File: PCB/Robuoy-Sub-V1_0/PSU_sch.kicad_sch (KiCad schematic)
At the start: 27 parts, among them U1 TPS5430DDAR, U7 TLV61046ADB, U8 TLV61046ADB

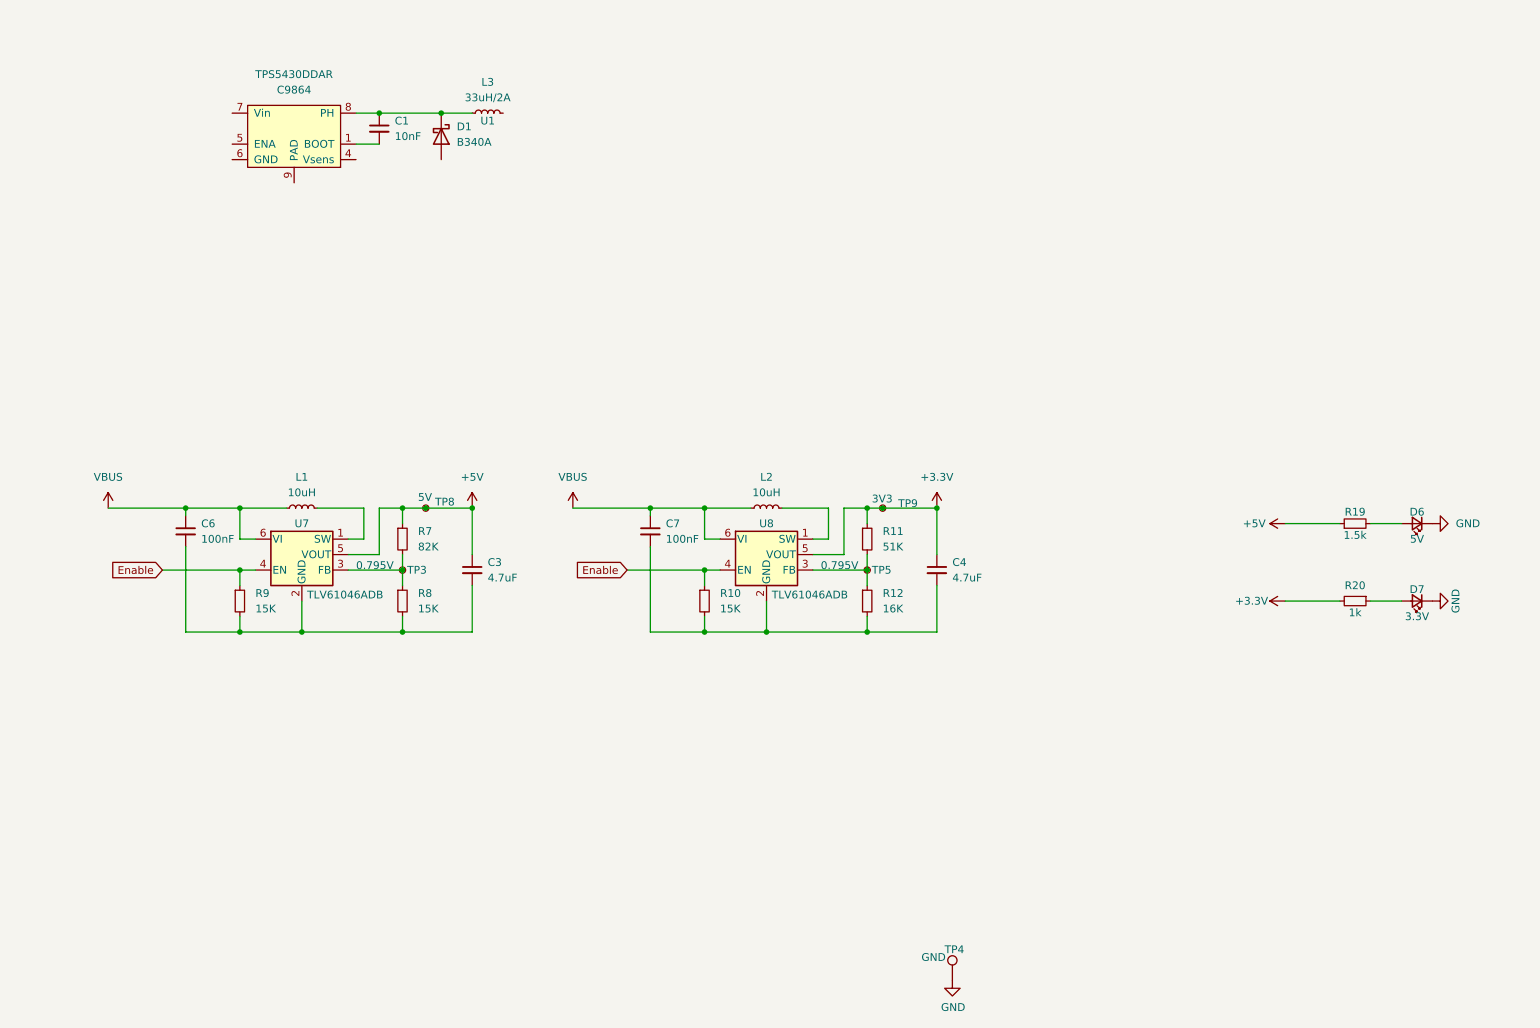
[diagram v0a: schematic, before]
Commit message: Schematic changes not yet finished!
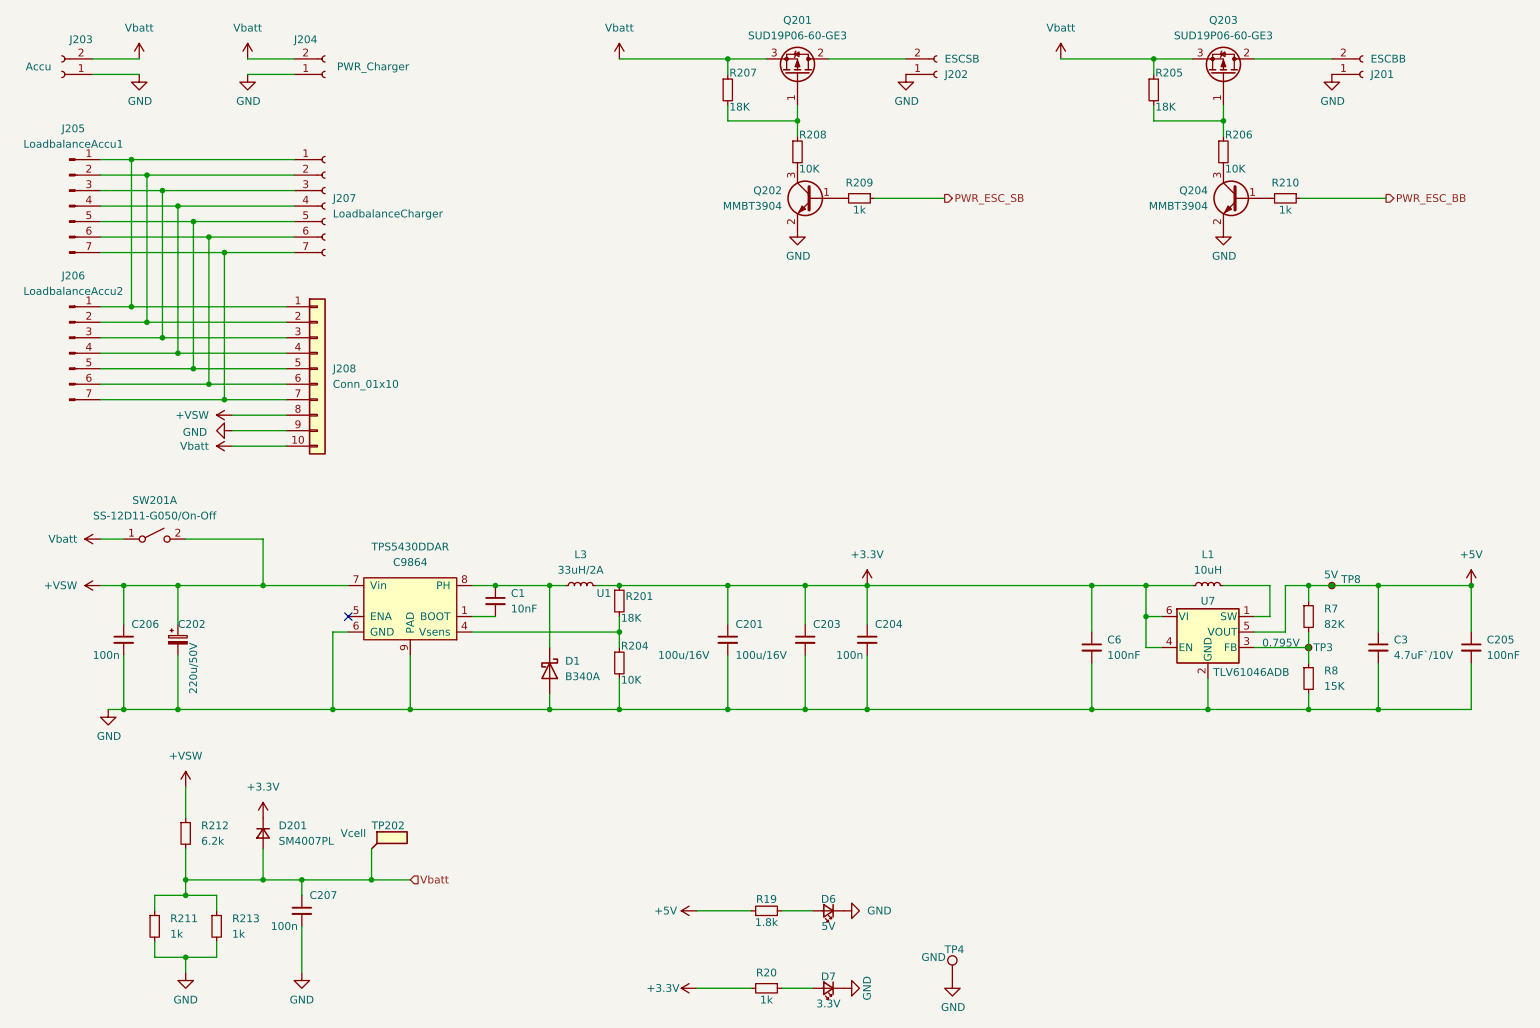
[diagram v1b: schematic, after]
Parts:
- removed C4: 4.7uF, symbol Device:C_Small
- removed C7: 100nF, symbol Device:C_Small
- removed L2: 10uH, symbol Device:L_Small
- removed R10, R9: 15K, symbol Device:R_Small
- removed R11: 51K, symbol Device:R_Small
- removed R12: 16K, symbol Device:R_Small
- removed TP5: 0.795V, symbol Connector:TestPoint_Small
- removed TP9: 3V3, symbol Connector:TestPoint_Small
- removed U8: TLV61046ADB, Package_TO_SOT_SMD:SOT-23-6, symbol Regulator_Switching:TLV61046ADB
- added C201, C203: 100u/16V, Capacitor_SMD:C_1210_3225Metric, symbol Device:C_Small
- added C202: 220u/50V, A_Device:CP_ALU_D10x10.5, symbol Device:C_Polarized_Small
- added C204, C206, C207: 100n, A_Device:C_0603, symbol Device:C_Small
- added C205: 100nF, symbol Device:C_Small
- added D201: SM4007PL, A_Device:D_SOD-123_2.85x1.8x1.3, symbol Device:D_Small
- added J201: ESCBB, symbol Connector:Conn_01x02_Socket
- added J202: ESCSB, symbol Connector:Conn_01x02_Socket
- added J203: Accu, A_Connector:AMASS_XT60-M_1x02_P7.20mm_Vertical, symbol Connector:Conn_01x02_Socket
- added J204: PWR_Charger, A_Connector:AMASS_XT60-M_1x02_P7.20mm_Vertical, symbol Connector:Conn_01x02_Socket
- added J205: LoadbalanceAccu1, symbol Connector:Conn_01x07_Pin
- added J206: LoadbalanceAccu2, symbol Connector:Conn_01x07_Pin
- added J207: LoadbalanceCharger, symbol Connector:Conn_01x07_Socket
- added J208: Conn_01x10, symbol Connector_Generic:Conn_01x10
- added Q201, Q203: SUD19P06-60-GE3, Package_TO_SOT_SMD:TO-252-2, symbol Transistor_FET:SUD19P06-60
- added Q202, Q204: MMBT3904, Package_TO_SOT_SMD:SOT-23, symbol Transistor_BJT:MMBT3904
- added R201, R205, R207: 18K, symbol Device:R_Small
- added R204, R206, R208: 10K, symbol Device:R_Small
- added R209, R210, R211, R213: 1k, A_Device:R_0603, symbol Device:R_Small
- added R212: 6.2k, A_Device:R_0603, symbol Device:R_Small
- added SW201: SS-12D11-G050/On-Off, symbol Switch:SW_DPST_x2
- added TP202: Vcell, A_Pads_Pins:Testpoint_0.6x1.0, symbol Connector:TestPoint_Flag
- C3: value 4.7uF -> 4.7uF`/10V
- R19: value 1.5k -> 1.8k; LCSC C22843 -> (none)
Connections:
- net Enable is gone; now on net +3.3V: U7.4 (EN)
- net VBUS is gone; now on net +3.3V: C6.1, L1.1, U7.6 (VI)
- net +3.3V: now also L3.2, C201.1, C203.1, C204.1, D201.1 (K), R201.1
- net +5V: now also C205.1
- net GND: now also C3.2, C6.2, D1.2 (A), R8.2, U1.6 (GND), U1.9 (PAD), U7.2 (GND), C201.2, C202.2, C203.2, C204.2, C205.2, C206.2, C207.2, J201.1 (Pin_1), J202.1 (Pin_1), J203.1 (Pin_1), J204.1 (Pin_1), J208.9 (Pin_9), Q202.2 (E), Q204.2 (E), R204.2, R211.2, R213.2
- net at U1.4 (Vsens): now also R201.2, R204.1
- net +VSW: now reaches U1.7 (Vin)
- net +VSW: now also C202.1, C206.1, J208.8 (Pin_8), R212.1, SW201.2 (B)
- new net: J201.2 (Pin_2), Q203.2 (D)
- new net: Q204.1 (B), R210.2
- new net: J205.1 (Pin_1), J206.1 (Pin_1), J207.1 (Pin_1), J208.1 (Pin_1)
- new net: J205.2 (Pin_2), J206.2 (Pin_2), J207.2 (Pin_2), J208.2 (Pin_2)
- new net: J205.3 (Pin_3), J206.3 (Pin_3), J207.3 (Pin_3), J208.3 (Pin_3)
- new net: J205.4 (Pin_4), J206.4 (Pin_4), J207.4 (Pin_4), J208.4 (Pin_4)
- new net: J205.5 (Pin_5), J206.5 (Pin_5), J207.5 (Pin_5), J208.5 (Pin_5)
- new net: J205.6 (Pin_6), J206.6 (Pin_6), J207.6 (Pin_6), J208.6 (Pin_6)
- new net: J205.7 (Pin_7), J206.7 (Pin_7), J207.7 (Pin_7), J208.7 (Pin_7)
- new net: Q202.1 (B), R209.2
- new net: Q202.3 (C), R208.2
- new net: J202.2 (Pin_2), Q201.2 (D)
- new net: Q203.1 (G), R205.2, R206.1
- new net: Q204.3 (C), R206.2
- new net: Q201.1 (G), R207.2, R208.1
- new net PWR_ESC_BB: R210.1
- new net PWR_ESC_SB: R209.1
- new net Vbatt: C207.1, D201.2 (A), J203.2 (Pin_2), J204.2 (Pin_2), J208.10 (Pin_10), Q201.3 (S), Q203.3 (S), R205.1, R207.1, R211.1, R212.2, R213.1, SW201.1 (A), TP202.1
- no-connect marks 0 -> 1
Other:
- moved on the sheet: C1, C3, C6, D1, D6, D7, L1, L3, R19, R20, R7, R8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
